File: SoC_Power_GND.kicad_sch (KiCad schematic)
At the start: 4 parts, among them U1 rv1126/rv1109, U2 rv1126/rv1109

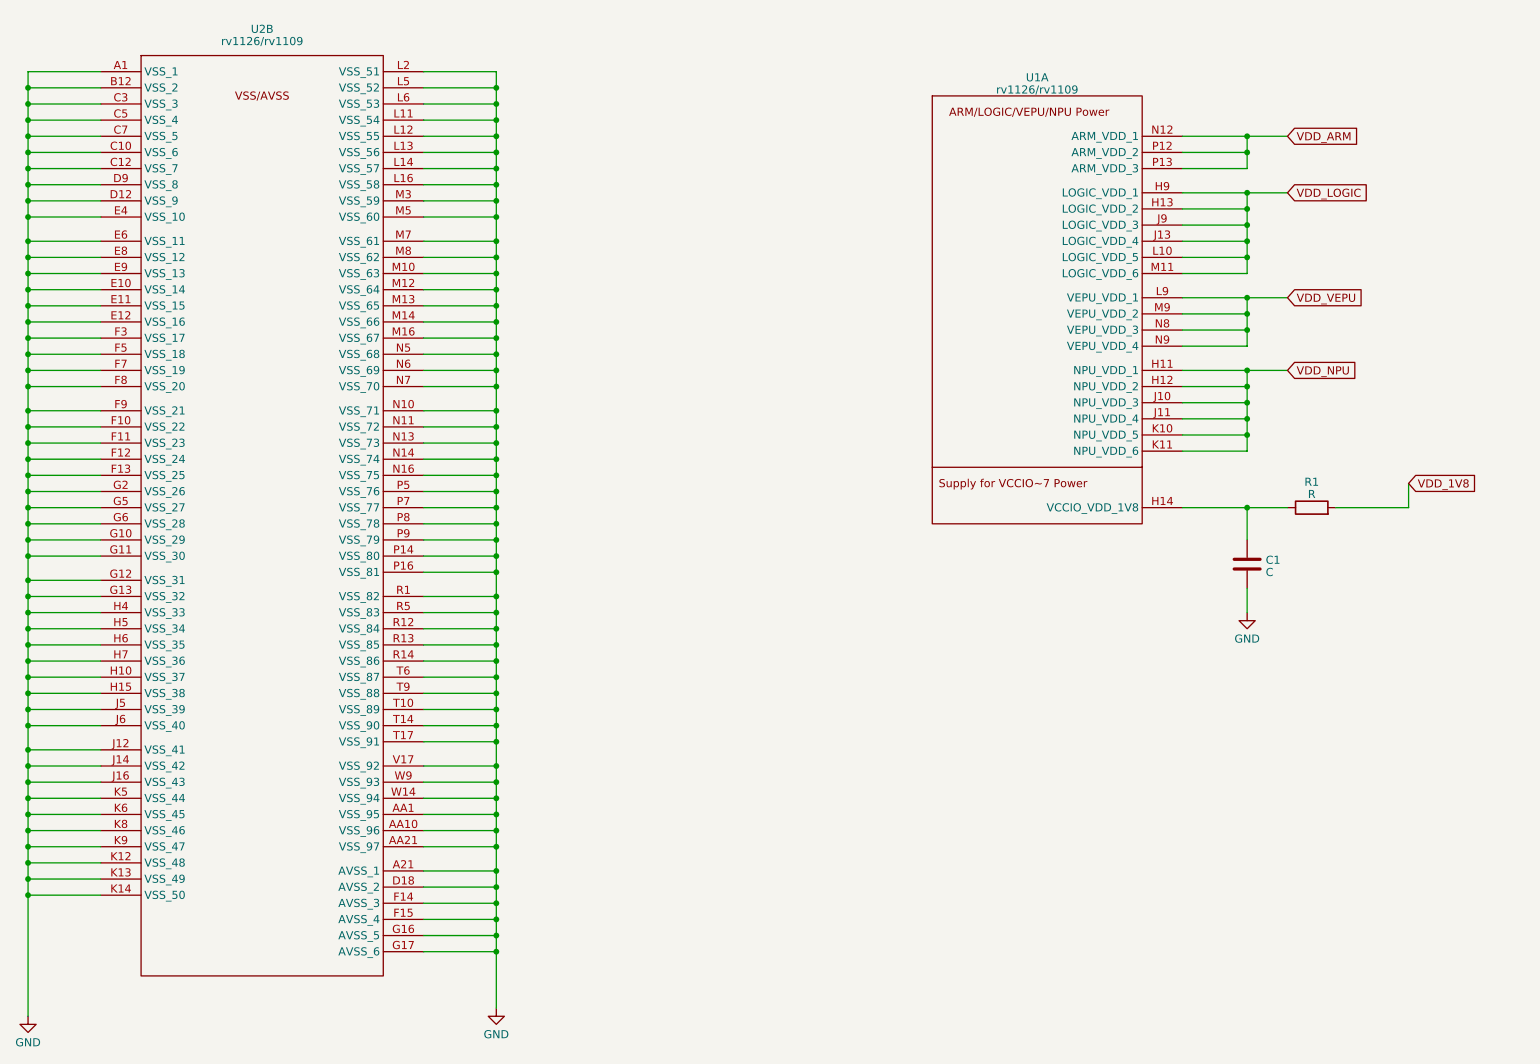
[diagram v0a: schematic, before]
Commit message: PMIC management
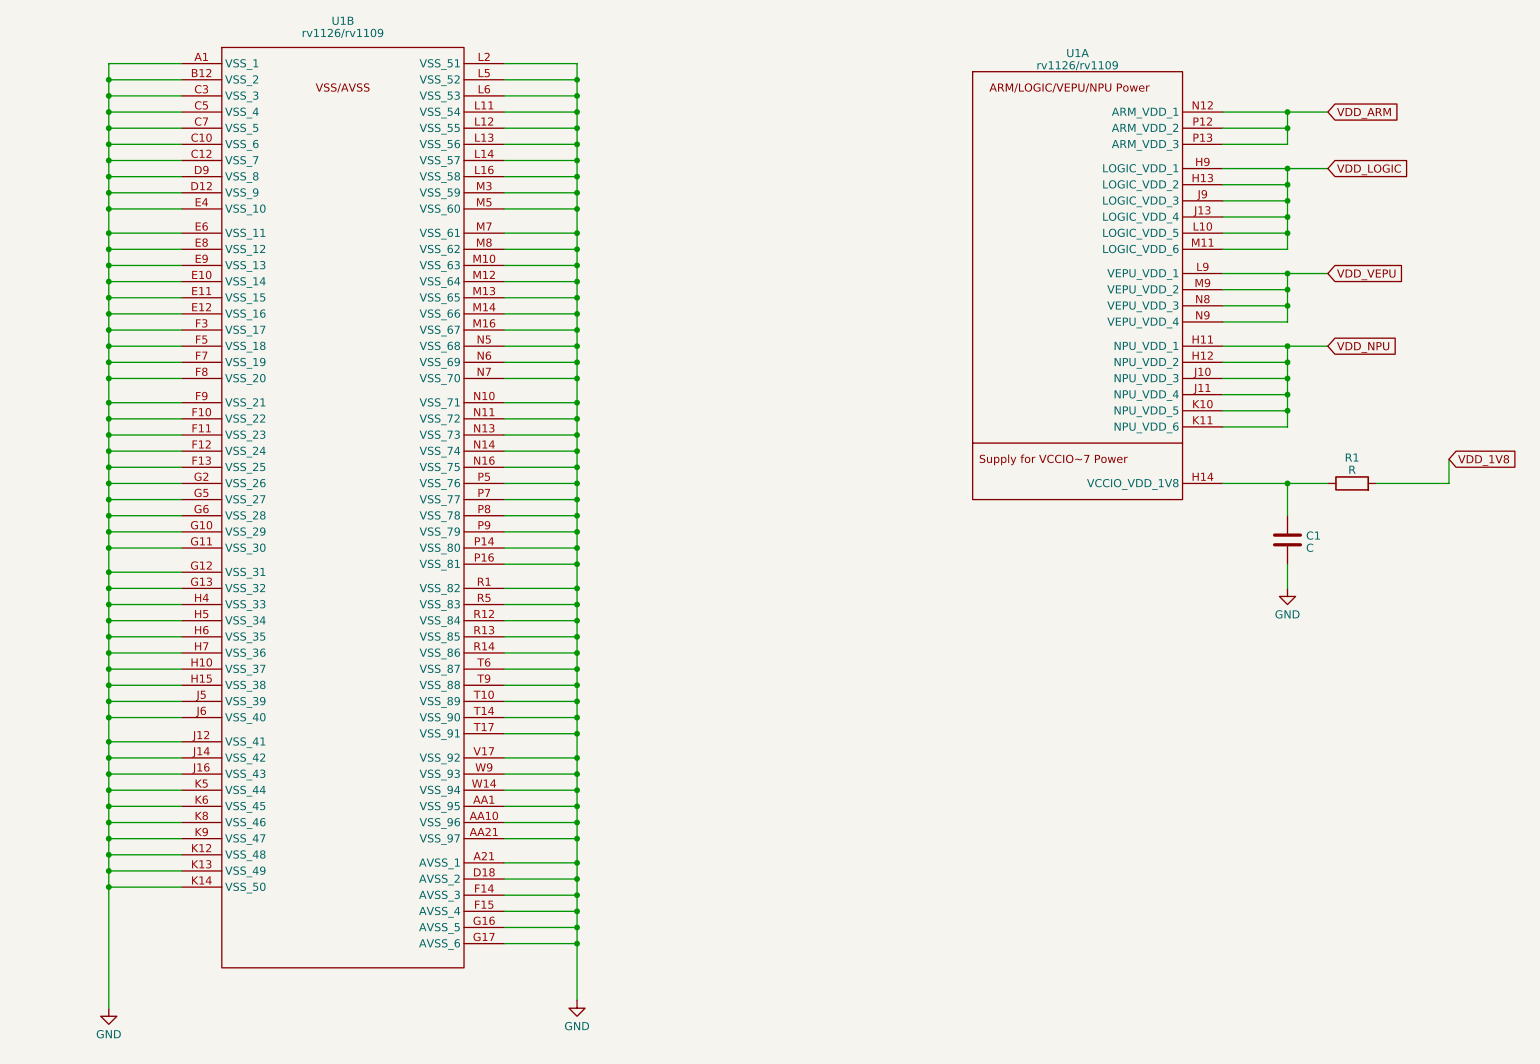
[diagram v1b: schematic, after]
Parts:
- removed U2: rv1126/rv1109, symbol CPU_Rockchip:rv1126_rv1109
- added unit 2 of U1
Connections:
- net GND: now also U1.A1 (VSS_1), U1.A21 (AVSS_1), U1.AA1 (VSS_95), U1.AA10 (VSS_96), U1.AA21 (VSS_97), U1.B12 (VSS_2), U1.C10 (VSS_6), U1.C12 (VSS_7), U1.C3 (VSS_3), U1.C5 (VSS_4), U1.C7 (VSS_5), U1.D12 (VSS_9), U1.D18 (AVSS_2), U1.D9 (VSS_8), U1.E10 (VSS_14), U1.E11 (VSS_15), U1.E12 (VSS_16), U1.E4 (VSS_10), U1.E6 (VSS_11), U1.E8 (VSS_12), U1.E9 (VSS_13), U1.F10 (VSS_22), U1.F11 (VSS_23), U1.F12 (VSS_24), U1.F13 (VSS_25), U1.F14 (AVSS_3), U1.F15 (AVSS_4), U1.F3 (VSS_17), U1.F5 (VSS_18), U1.F7 (VSS_19), U1.F8 (VSS_20), U1.F9 (VSS_21), U1.G10 (VSS_29), U1.G11 (VSS_30), U1.G12 (VSS_31), U1.G13 (VSS_32), U1.G16 (AVSS_5), U1.G17 (AVSS_6), U1.G2 (VSS_26), U1.G5 (VSS_27), U1.G6 (VSS_28), U1.H10 (VSS_37), U1.H15 (VSS_38), U1.H4 (VSS_33), U1.H5 (VSS_34), U1.H6 (VSS_35), U1.H7 (VSS_36), U1.J12 (VSS_41), U1.J14 (VSS_42), U1.J16 (VSS_43), U1.J5 (VSS_39), U1.J6 (VSS_40), U1.K12 (VSS_48), U1.K13 (VSS_49), U1.K14 (VSS_50), U1.K5 (VSS_44), U1.K6 (VSS_45), U1.K8 (VSS_46), U1.K9 (VSS_47), U1.L11 (VSS_54), U1.L12 (VSS_55), U1.L13 (VSS_56), U1.L14 (VSS_57), U1.L16 (VSS_58), U1.L2 (VSS_51), U1.L5 (VSS_52), U1.L6 (VSS_53), U1.M10 (VSS_63), U1.M12 (VSS_64), U1.M13 (VSS_65), U1.M14 (VSS_66), U1.M16 (VSS_67), U1.M3 (VSS_59), U1.M5 (VSS_60), U1.M7 (VSS_61), U1.M8 (VSS_62), U1.N10 (VSS_71), U1.N11 (VSS_72), U1.N13 (VSS_73), U1.N14 (VSS_74), U1.N16 (VSS_75), U1.N5 (VSS_68), U1.N6 (VSS_69), U1.N7 (VSS_70), U1.P14 (VSS_80), U1.P16 (VSS_81), U1.P5 (VSS_76), U1.P7 (VSS_77), U1.P8 (VSS_78), U1.P9 (VSS_79), U1.R1 (VSS_82), U1.R12 (VSS_84), U1.R13 (VSS_85), U1.R14 (VSS_86), U1.R5 (VSS_83), U1.T10 (VSS_89), U1.T14 (VSS_90), U1.T17 (VSS_91), U1.T6 (VSS_87), U1.T9 (VSS_88), U1.V17 (VSS_92), U1.W14 (VSS_94), U1.W9 (VSS_93)
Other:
- company: Qingdao IotPi Information Technology -> (none)
- title: Leaf RV1126 Power -> (none)

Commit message: PMIC DCDC
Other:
- company: (none) -> Qingdao IotPi Information Technology
- title: (none) -> Leaf RV1126 PMIC RK809
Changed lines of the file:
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@@
 (kicad_sch (version 20230121) (generator eeschema)
   (paper "A4")
+  (title_block
+    (title "Leaf RV1126 PMIC RK809")
+    (date "2023-02-23")
+    (rev "1")
+    (company "Qingdao IotPi Information Technology")
+  )
   (junction (at 43.18 38.1) (diameter 0) (color 0 0 0 0)
   )

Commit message: updated: PMIC codec
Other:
- title: Leaf RV1126 PMIC RK809 -> Leaf RV1126 PMIC RK809 Codec
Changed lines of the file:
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@@
   (paper "A4")
   (title_block
-    (title "Leaf RV1126 PMIC RK809")
-    (date "2023-02-23")
+    (title "Leaf RV1126 PMIC RK809 Codec")
+    (date "2023-02-25")
     (rev "1")
     (company "Qingdao IotPi Information Technology")

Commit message: updated: titles
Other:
- title: Leaf RV1126 PMIC RK809 Codec -> Leaf RV1126 RK809 SoC Power
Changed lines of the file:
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@@
   (paper "A4")
   (title_block
-    (title "Leaf RV1126 PMIC RK809 Codec")
+    (title "Leaf RV1126 RK809 SoC Power")
     (date "2023-02-25")
     (rev "1")
